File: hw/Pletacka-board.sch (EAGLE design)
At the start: 29 parts, among them U1 LM75BDP

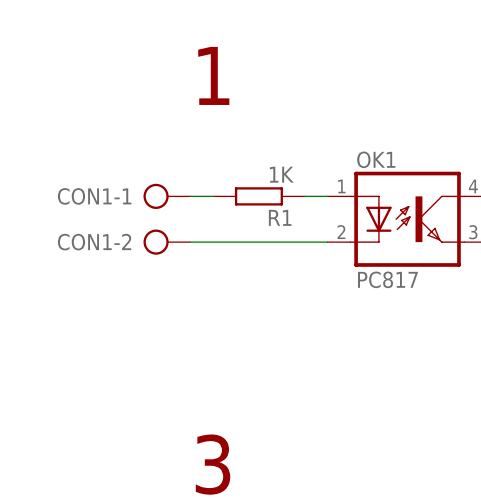
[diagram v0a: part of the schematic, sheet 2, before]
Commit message: Start routing
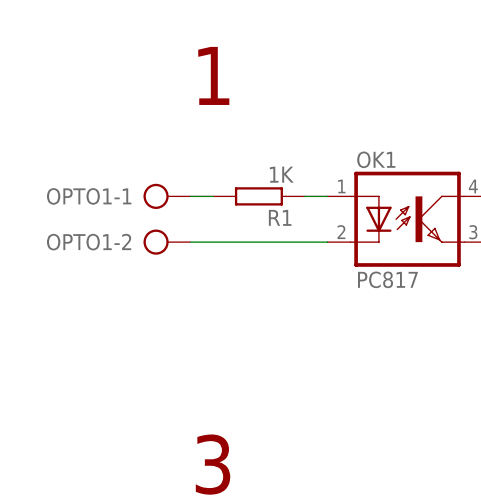
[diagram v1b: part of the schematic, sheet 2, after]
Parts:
- renumbered CON1 to OPTO1
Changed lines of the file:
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@@
 <part name="FRAME2" library="frames" library_urn="urn:adsk.eagle:library:229" deviceset="A4L-LOC" device=""/>
 <part name="U$1" library="ESP32-T-Display" deviceset="ESP-32-T-DISPLAY" device=""/>
-<part name="CON1" library="#Svorkovnice" deviceset="AK500/2" device=""/>
+<part name="OPTO1" library="#Svorkovnice" deviceset="AK500/2" device=""/>
 <part name="RDM1" library="RDM6300" deviceset="RDM6300" device=""/>
 <part name="+3V2" library="supply1" library_urn="urn:adsk.eagle:library:371" deviceset="+3V3" device=""/>
@@
 <attribute name="SHEET" x="230.505" y="5.08" size="2.54" layer="94"/>
 </instance>
-<instance part="CON1" gate="-1" x="27.94" y="142.24" smashed="yes">
+<instance part="OPTO1" gate="-1" x="27.94" y="142.24" smashed="yes">
 <attribute name="NAME" x="26.67" y="143.129" size="1.778" layer="95" rot="R180"/>
 </instance>
-<instance part="CON1" gate="-2" x="27.94" y="137.16" smashed="yes">
+<instance part="OPTO1" gate="-2" x="27.94" y="137.16" smashed="yes">
 <attribute name="NAME" x="26.67" y="138.049" size="1.778" layer="95" rot="R180"/>
 <attribute name="VALUE" x="24.13" y="133.477" size="1.778" layer="96"/>
@@
 <net name="N$2" class="0">
 <segment>
-<pinref part="CON1" gate="-2" pin="KL"/>
+<pinref part="OPTO1" gate="-2" pin="KL"/>
 <pinref part="OK1" gate="A" pin="C"/>
 <wire x1="33.02" y1="137.16" x2="48.26" y2="137.16" width="0.1524" layer="91"/>
@@
 <net name="N$4" class="0">
 <segment>
-<pinref part="CON1" gate="-1" pin="KL"/>
+<pinref part="OPTO1" gate="-1" pin="KL"/>
 <pinref part="R1" gate="G$1" pin="2"/>
 <wire x1="33.02" y1="142.24" x2="35.56" y2="142.24" width="0.1524" layer="91"/>
